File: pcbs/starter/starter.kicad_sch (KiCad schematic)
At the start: 17 parts, among them J1 Conn_01x06_Socket, J2 Relay Anschluss, J3 12V Eingang und GND, J4 Conn_01x02_Socket, Q2 2N7000, Q3 2N7000, Q4 2N7000, U1 ESP32-C3_SUPERMINI_TH

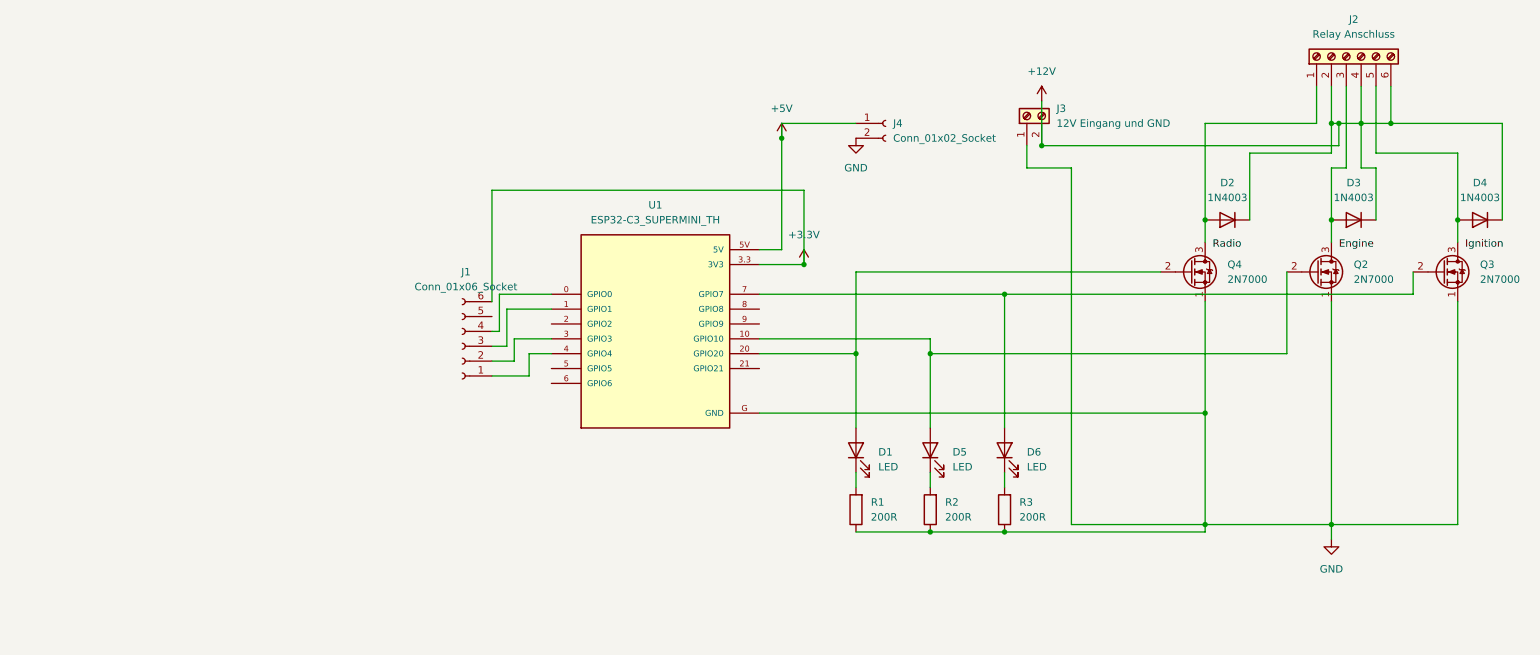
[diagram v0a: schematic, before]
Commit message: first pcb revision ordered at JLCPCB
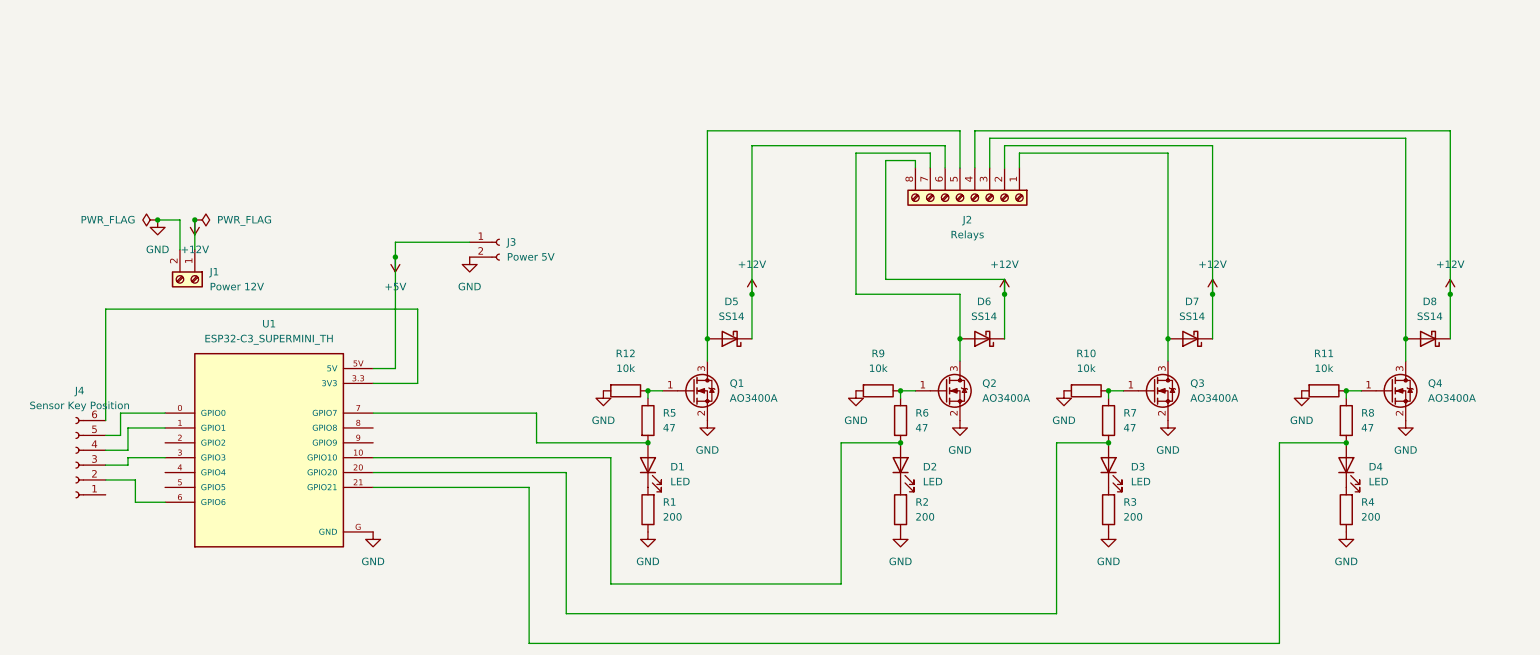
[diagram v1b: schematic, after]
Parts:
- removed D2, D3, D4: 1N4003, Diode_THT:D_DO-41_SOD81_P10.16mm_Horizontal, symbol Diode:1N4003
- removed D5, D6: LED, LED_THT:LED_D5.0mm, symbol Device:LED
- removed J2: Relay Anschluss, TerminalBlock_CUI:TerminalBlock_CUI_TB007-508-06_1x06_P5.08mm_Horizontal, symbol Connector:Screw_Terminal_01x06
- removed Q2, Q3, Q4: 2N7000, Package_TO_SOT_THT:TO-92_Inline, symbol Transistor_FET:2N7000
- added D2, D3, D4: LED, LED_SMD:LED_0805_2012Metric_Pad1.15x1.40mm_HandSolder, symbol Device:LED
- added D5, D6, D7, D8: SS14, Diode_SMD:D_SMA, symbol Diode:SS14
- added J2: Relays, TerminalBlock_Phoenix:TerminalBlock_Phoenix_MKDS-1,5-8-5.08_1x08_P5.08mm_Horizontal, symbol Connector:Screw_Terminal_01x08
- added Q1, Q2, Q3, Q4: AO3400A, Package_TO_SOT_SMD:SOT-23, symbol Transistor_FET:AO3400A
- added R10, R11, R12, R9: 10k, Resistor_SMD:R_1206_3216Metric_Pad1.30x1.75mm_HandSolder, symbol Device:R
- added R4: 200, Resistor_SMD:R_1206_3216Metric_Pad1.30x1.75mm_HandSolder, symbol Device:R
- added R5, R6, R7, R8: 47, Resistor_SMD:R_1206_3216Metric_Pad1.30x1.75mm_HandSolder, symbol Device:R
- D1: footprint LED_THT:LED_D5.0mm -> LED_SMD:LED_0805_2012Metric_Pad1.15x1.40mm_HandSolder
- J1: renamed from J3; value 12V Eingang und GND -> Power 12V; footprint TerminalBlock_CUI:TerminalBlock_CUI_TB007-508-02_1x02_P5.08mm_Horizontal -> TerminalBlock_Phoenix:TerminalBlock_Phoenix_MKDS-1,5-2-5.08_1x02_P5.08mm_Horizontal
- J3: renamed from J4; value Conn_01x02_Socket -> Power 5V; footprint Connector_JST:JST_XH_B2B-XH-AM_1x02_P2.50mm_Vertical -> Connector_JST:JST_XH_B2B-XH-A_1x02_P2.50mm_Vertical
- J4: renamed from J1; value Conn_01x06_Socket -> Sensor Key Position; footprint Connector_JST:JST_XH_B6B-XH-AM_1x06_P2.50mm_Vertical -> Connector_JST:JST_XH_B6B-XH-A_1x06_P2.50mm_Vertical
- R1, R2, R3: value 200R -> 200; footprint Resistor_THT:R_Axial_DIN0204_L3.6mm_D1.6mm_P5.08mm_Horizontal -> Resistor_SMD:R_1206_3216Metric_Pad1.30x1.75mm_HandSolder
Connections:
- net +12V: now also J1.1 (Pin_1), D5.1 (K), D6.1 (K), D7.1 (K), D8.1 (K), J2.2 (Pin_2), J2.4 (Pin_4), J2.6 (Pin_6), J2.8 (Pin_8); no longer J1.2 (Pin_2)
- net GND: now also J1.2 (Pin_2), Q1.2 (S), Q2.2 (S), Q3.2 (S), Q4.2 (S), R10.2, R11.2, R12.2, R4.1, R9.2; no longer J1.1 (Pin_1)
- net at R2.2: now also D2.1 (K)
- net at J4.1 (Pin_1): no longer U1.4 (GPIO4)
- net at J4.2 (Pin_2): now also U1.6 (GPIO6); no longer U1.3 (GPIO3)
- net at J4.3 (Pin_3): now also U1.3 (GPIO3); no longer U1.1 (GPIO1)
- net at J4.4 (Pin_4): now also U1.1 (GPIO1); no longer U1.0 (GPIO0)
- net at J4.5 (Pin_5): now also U1.0 (GPIO0)
- net at D1.2 (A): now also U1.7 (GPIO7), R5.2; no longer U1.20 (GPIO20)
- net at U1.10 (GPIO10): now also D2.2 (A), R6.2
- net at R3.2: now also D3.1 (K)
- net at U1.21 (GPIO21): now also D4.2 (A), R8.2
- net +3.3V: no longer names the net of J4.6 (Pin_6), U1.3.3 (3V3)
- new net: Q3.1 (G), R10.1, R7.1
- new net: D8.2 (A), J2.3 (Pin_3), Q4.3 (D)
- new net: D7.2 (A), J2.1 (Pin_1), Q3.3 (D)
- new net: Q1.1 (G), R12.1, R5.1
- new net: D5.2 (A), J2.5 (Pin_5), Q1.3 (D)
- new net: D6.2 (A), J2.7 (Pin_7), Q2.3 (D)
- new net: Q2.1 (G), R6.1, R9.1
- new net: Q4.1 (G), R11.1, R8.1
- new net: D3.2 (A), R7.2, U1.20 (GPIO20)
- new net: D4.1 (K), R4.2
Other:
- moved on the sheet: D1, J1, J3, J4, R1, U1
